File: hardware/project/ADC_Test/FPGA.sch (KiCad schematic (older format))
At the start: 64 parts, among them J801 Conn_01x04_Male, J802 Conn_02x05, Q801 BC857, U801 SN74LVC1T45DBV, U802 SN74LVC1T45DBV, U803 ICE40HX4K-TQ144, U804 SN74LVC1T45DBV, U805 SN74LVC1T45DBV, U806 SN74LVC1T45DBV, U807 SN74LVC1T45DBV, U808 ASDMB-100.000MHZ, U809 MT25QL128ABA1ESE

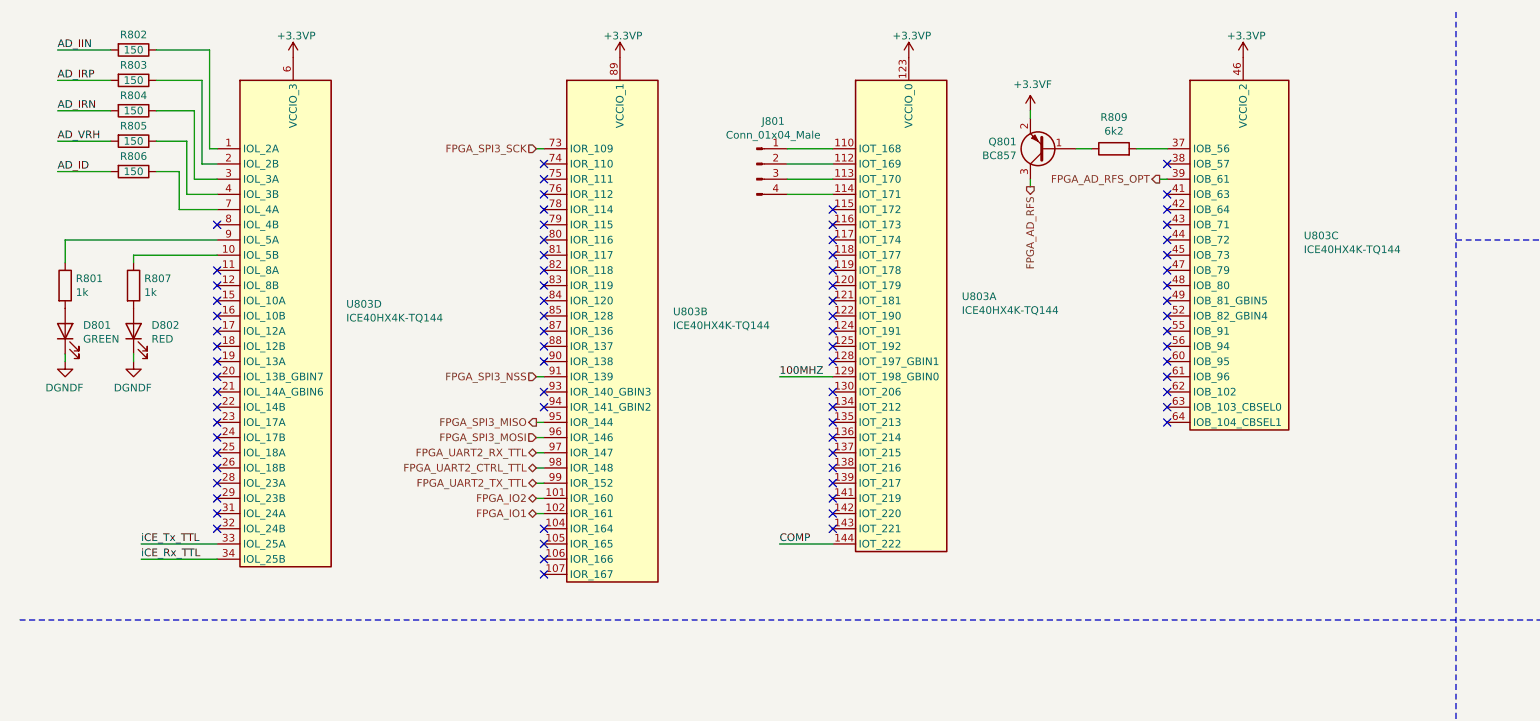
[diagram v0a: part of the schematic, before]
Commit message: PCB design.
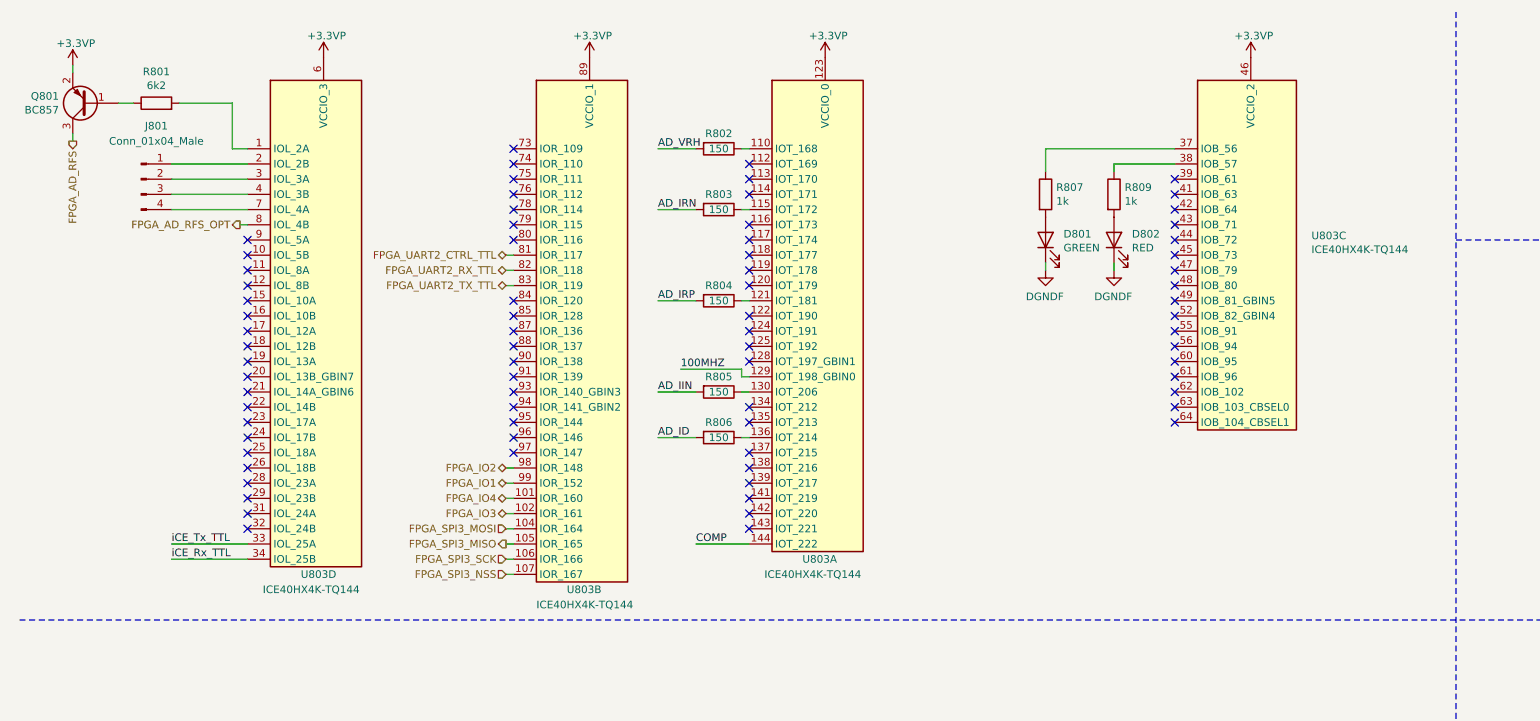
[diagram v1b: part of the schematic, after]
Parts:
- renumbered R809 to R801, R805 to R802, R804 to R803, R803 to R804, R802 to R805, R801 to R807, R807 to R809
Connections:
- net +3.3VF is gone; now on net +3.3VP: Q801.2 (E)
- net FPGA_AD_RFS_OPT: now also U803.8 (IOL_4B); no longer U803.39 (IOB_61)
- net FPGA_IO1: now also U803.99 (IOR_152); no longer U803.102 (IOR_161)
- net FPGA_IO2: now also U803.98 (IOR_148); no longer U803.101 (IOR_160)
- net FPGA_SPI3_MISO: now also U803.105 (IOR_165); no longer U803.95 (IOR_144)
- net FPGA_SPI3_MOSI: now also U803.104 (IOR_164); no longer U803.96 (IOR_146)
- net FPGA_SPI3_NSS: now also U803.107 (IOR_167); no longer U803.91 (IOR_139)
- net FPGA_SPI3_SCK: now also U803.106 (IOR_166); no longer U803.73 (IOR_109)
- net FPGA_UART2_CTRL_TTL: now also U803.81 (IOR_117); no longer U803.98 (IOR_148)
- net FPGA_UART2_RX_TTL: now also U803.82 (IOR_118); no longer U803.97 (IOR_147)
- net FPGA_UART2_TX_TTL: now also U803.83 (IOR_119); no longer U803.99 (IOR_152)
- net at R806.1: now also U803.136 (IOT_214); no longer U803.7 (IOL_4A)
- net at R802.1: now also U803.110 (IOT_168); no longer U803.4 (IOL_3B)
- net at R803.1: now also U803.115 (IOT_172); no longer U803.3 (IOL_3A)
- net at R804.1: now also U803.121 (IOT_181); no longer U803.2 (IOL_2B)
- net at R805.1: now also U803.130 (IOT_206); no longer U803.1 (IOL_2A)
- net at R809.1: now also U803.38 (IOB_57); no longer U803.10 (IOL_5B)
- net at R807.1: now also U803.37 (IOB_56); no longer U803.9 (IOL_5A)
- net at J801.1 (Pin_1): now also U803.2 (IOL_2B); no longer U803.110 (IOT_168)
- net at U803.112 (IOT_169): no longer J801.2 (Pin_2)
- net at U803.113 (IOT_170): no longer J801.3 (Pin_3)
- net at U803.114 (IOT_171): no longer J801.4 (Pin_4)
- net at R801.2: now also U803.1 (IOL_2A); no longer U803.37 (IOB_56)
- new net: J801.2 (Pin_2), U803.3 (IOL_3A)
- new net: J801.3 (Pin_3), U803.4 (IOL_3B)
- new net: J801.4 (Pin_4), U803.7 (IOL_4A)
- new net FPGA_IO3: U803.102 (IOR_161)
- new net FPGA_IO4: U803.101 (IOR_160)
- no-connect marks 79 -> 77
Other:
- moved on the sheet: D801, D802, J801, Q801, R801, R802, R803, R804, R805, R806, R807, R809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
